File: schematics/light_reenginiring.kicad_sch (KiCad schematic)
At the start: 13 parts, among them SW1 SW_SPDT, U1 MB10F

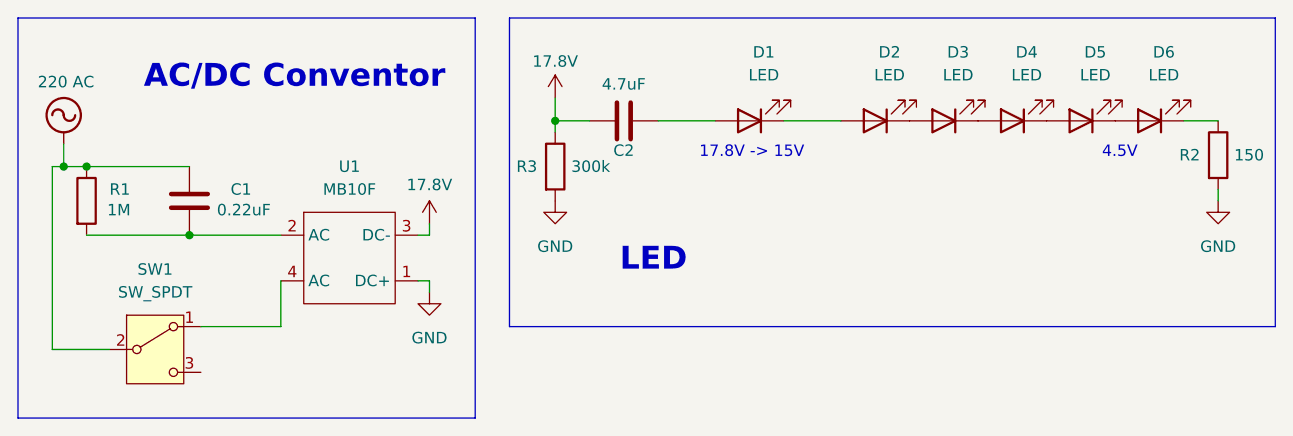
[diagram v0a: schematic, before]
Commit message: fix schematic
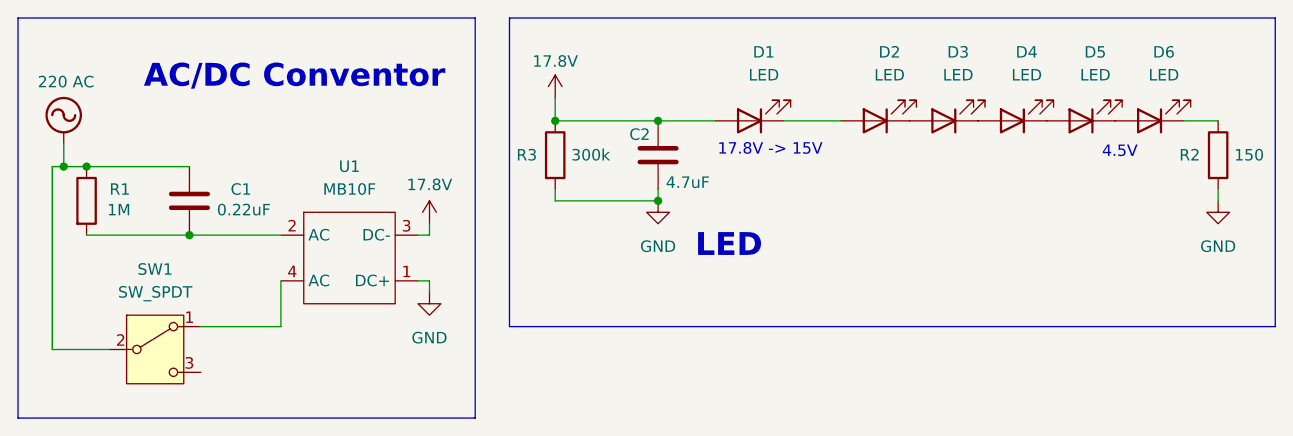
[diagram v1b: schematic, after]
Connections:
- net 17.8V: now also D1.2 (A)
- net GND: now also C2.2
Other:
- moved on the sheet: C2, R3
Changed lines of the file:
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@@
 	(text "17.8V -> 15V"
 		(exclude_from_sim no)
-		(at 99.314 32.766 0)
+		(at 101.346 32.512 0)
 		(effects
 			(font
@@
 	(text "LED"
 		(exclude_from_sim no)
-		(at 88.392 44.704 0)
+		(at 96.774 43.18 0)
 		(effects
 			(font
@@
 	)
 	(junction
+		(at 88.9 29.21)
+		(diameter 0)
+		(color 0 0 0 0)
+	)
+	(junction
 		(at 36.83 41.91)
 		(diameter 0)
@@
 	)
 	(junction
+		(at 88.9 38.1)
+		(diameter 0)
+		(color 0 0 0 0)
+	)
+	(junction
 		(at 77.47 29.21)
 		(diameter 0)
@@
 	(wire
 		(pts
-			(xy 77.47 29.21) (xy 77.47 30.48)
-		)
-		(stroke
-			(width 0)
-			(type default)
-		)
-	)
-	(wire
-		(pts
 			(xy 46.99 52.07) (xy 46.99 46.99)
 		)
@@
 	(wire
 		(pts
-			(xy 81.28 29.21) (xy 77.47 29.21)
+			(xy 77.47 29.21) (xy 88.9 29.21)
+		)
+		(stroke
+			(width 0)
+			(type default)
+		)
+	)
+	(wire
+		(pts
+			(xy 77.47 36.83) (xy 77.47 38.1)
 		)
 		(stroke
@@
 	(wire
 		(pts
+			(xy 88.9 36.83) (xy 88.9 38.1)
+		)
+		(stroke
+			(width 0)
+			(type default)
+		)
+	)
+	(wire
+		(pts
 			(xy 21.59 34.29) (xy 21.59 54.61)
 		)
@@
 	(wire
 		(pts
+			(xy 77.47 38.1) (xy 88.9 38.1)
+		)
+		(stroke
+			(width 0)
+			(type default)
+		)
+	)
+	(wire
+		(pts
 			(xy 63.5 46.99) (xy 63.5 48.26)
 		)
@@
 	(symbol
 		(lib_id "Device:C")
-		(at 85.09 29.21 90)
+		(at 88.9 33.02 0)
 		(unit 1)
 		(exclude_from_sim no)
@@
 		(dnp no)
 		(property "Reference" "C2"
-			(at 85.09 32.512 90)
+			(at 86.868 30.734 0)
 			(effects
 				(font
@@
 		)
 		(property "Value" "4.7uF"
-			(at 85.09 25.146 90)
-			(effects
-				(font
-					(size 1.27 1.27)
-				)
-			)
-		)
-		(property "Footprint" ""
-			(at 88.9 28.2448 0)
+			(at 92.202 36.068 0)
+			(effects
+				(font
+					(size 1.27 1.27)
+				)
+			)
+		)
+		(property "Footprint" ""
+			(at 89.8652 36.83 0)
 			(effects
 				(font
@@
 		)
 		(property "Datasheet" "~"
-			(at 85.09 29.21 0)
+			(at 88.9 33.02 0)
 			(effects
 				(font
@@
 		)
 		(property "Description" "Unpolarized capacitor"
-			(at 85.09 29.21 0)
+			(at 88.9 33.02 0)
 			(effects
 				(font
@@
 		)
 		(instances
-			(project ""
+			(project "light_reenginiring"
 				(path "/7bff3f35-c707-432f-a3d1-71506696911d"
 					(reference "C2")
@@
 	(symbol
 		(lib_id "Device:R")
-		(at 77.47 34.29 0)
+		(at 77.47 33.02 0)
 		(unit 1)
 		(exclude_from_sim no)
@@
 		(dnp no)
 		(property "Reference" "R3"
-			(at 73.152 34.29 0)
+			(at 73.152 33.02 0)
 			(effects
 				(font
@@
 		)
 		(property "Value" "300k"
-			(at 79.248 34.29 0)
+			(at 79.248 33.02 0)
 			(effects
 				(font
@@
 		)
 		(property "Footprint" ""
-			(at 75.692 34.29 90)
+			(at 75.692 33.02 90)
 			(effects
 				(font
@@
 		)
 		(property "Datasheet" "~"
-			(at 77.47 34.29 0)
+			(at 77.47 33.02 0)
 			(effects
 				(font
@@
 		)
 		(property "Description" "Resistor"
-			(at 77.47 34.29 0)
+			(at 77.47 33.02 0)
 			(effects
 				(font
@@
 	(symbol
 		(lib_id "power:GND")
-		(at 77.47 38.1 0)
+		(at 88.9 38.1 0)
 		(unit 1)
 		(exclude_from_sim no)
@@
 		(fields_autoplaced yes)
 		(property "Reference" "#PWR06"
-			(at 77.47 44.45 0)
+			(at 88.9 44.45 0)
 			(effects
 				(font
@@
 		)
 		(property "Value" "GND"
-			(at 77.47 43.18 0)
-			(effects
-				(font
-					(size 1.27 1.27)
-				)
-			)
-		)
-		(property "Footprint" ""
-			(at 77.47 38.1 0)
+			(at 88.9 43.18 0)
+			(effects
+				(font
+					(size 1.27 1.27)
+				)
+			)
+		)
+		(property "Footprint" ""
+			(at 88.9 38.1 0)
 			(effects
 				(font
@@
 		)
 		(property "Datasheet" ""
-			(at 77.47 38.1 0)
+			(at 88.9 38.1 0)
 			(effects
 				(font
@@
 		)
 		(property "Description" "Power symbol creates a global label with name \"GND\" , ground"
-			(at 77.47 38.1 0)
-			(effects
-				(font
+			(at 88.9 38.1 0)
+			(effects
+				(font
